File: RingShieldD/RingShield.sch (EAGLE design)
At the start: 28 parts

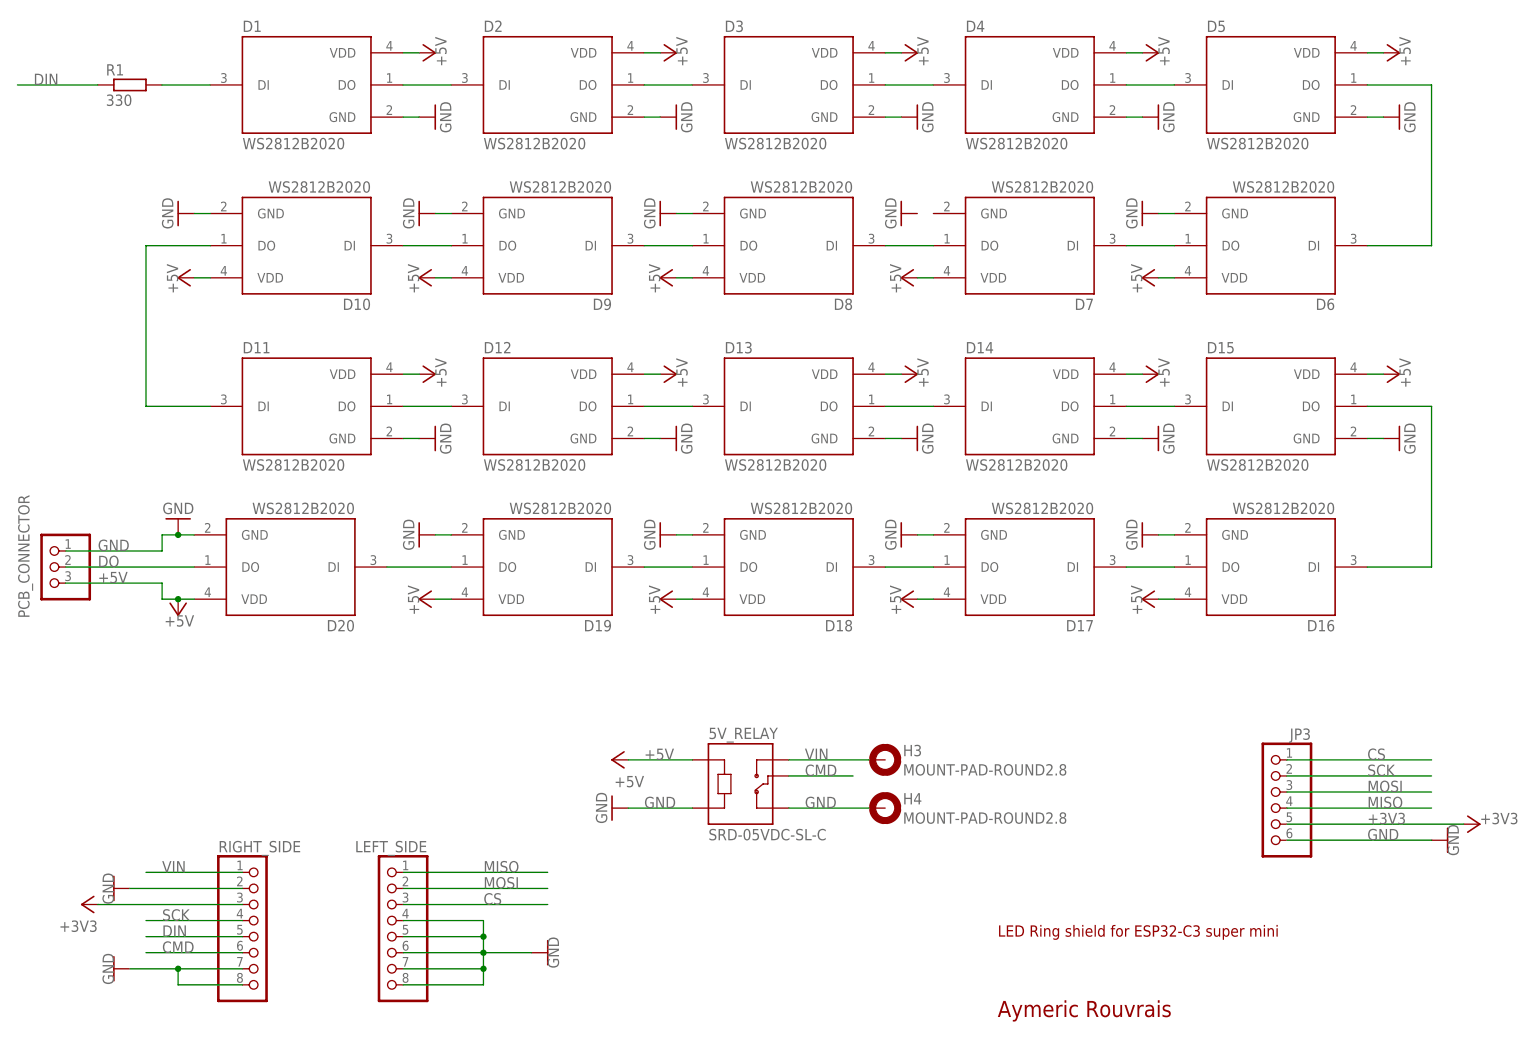
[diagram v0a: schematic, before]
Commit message: Chagnging right side
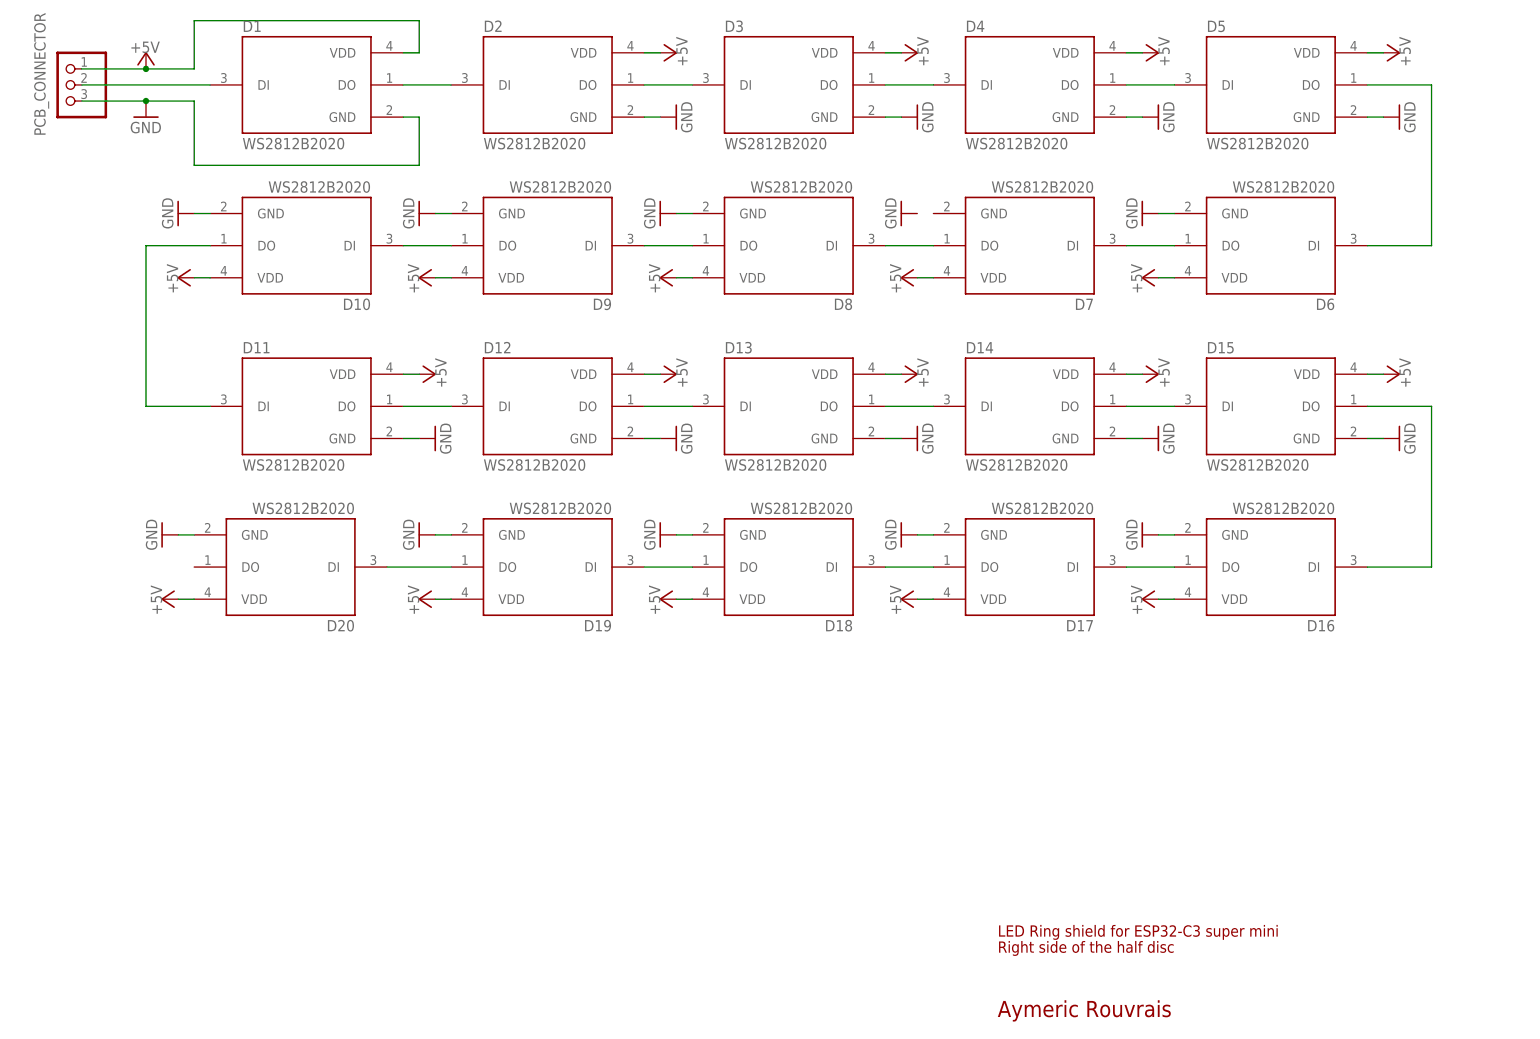
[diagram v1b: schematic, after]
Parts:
- removed 5V_RELAY: SRD-05VDC-SL-C, SRD-05VDC-SL-C:SRD-05VDC-SL-C
- removed H3, H4: MOUNT-PAD-ROUND2.8, holes:MOUNT-PAD-ROUND2.8
- removed JP3: (no value), pinhead:PINHD-1X6/90
- removed LEFT_SIDE, RIGHT_SIDE: (no value), pinhead:PINHD-1X8
- removed R1: 330, rcl:R-EU_0204/7
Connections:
- removed net +3V3: JP3.5, RIGHT_SIDE.3
- removed net CMD: 5V_RELAY.COM, RIGHT_SIDE.6
- removed net CS: JP3.1, LEFT_SIDE.3
- removed net DIN: R1.1, RIGHT_SIDE.5
- removed net DO: D20.DO, PCB_CONNECTOR.2
- removed net MISO: JP3.4, LEFT_SIDE.1
- removed net MOSI: JP3.3, LEFT_SIDE.2
- removed net SCK: JP3.2, RIGHT_SIDE.4
- removed net VIN: 5V_RELAY.NO, H3.MOUNT, RIGHT_SIDE.1
- net +5V: now also PCB_CONNECTOR.1; no longer 5V_RELAY.A1, PCB_CONNECTOR.3
- net GND: now also PCB_CONNECTOR.3; no longer 5V_RELAY.A2, 5V_RELAY.NC, H4.MOUNT, JP3.6, LEFT_SIDE.4, LEFT_SIDE.5, LEFT_SIDE.6, LEFT_SIDE.7, LEFT_SIDE.8, PCB_CONNECTOR.1, RIGHT_SIDE.2, RIGHT_SIDE.7, RIGHT_SIDE.8
- net N$1: now also PCB_CONNECTOR.2; no longer R1.2
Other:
- note added: "Right side of the half disc"
- note removed: "External power supply"
- moved on the sheet: PCB_CONNECTOR
